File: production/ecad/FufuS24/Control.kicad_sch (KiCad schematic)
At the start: 28 parts, among them IC1 NLVPCA9535EDTR2G, J2 Conn_01x02, U1 RP2040, U2 W25Q128JVS

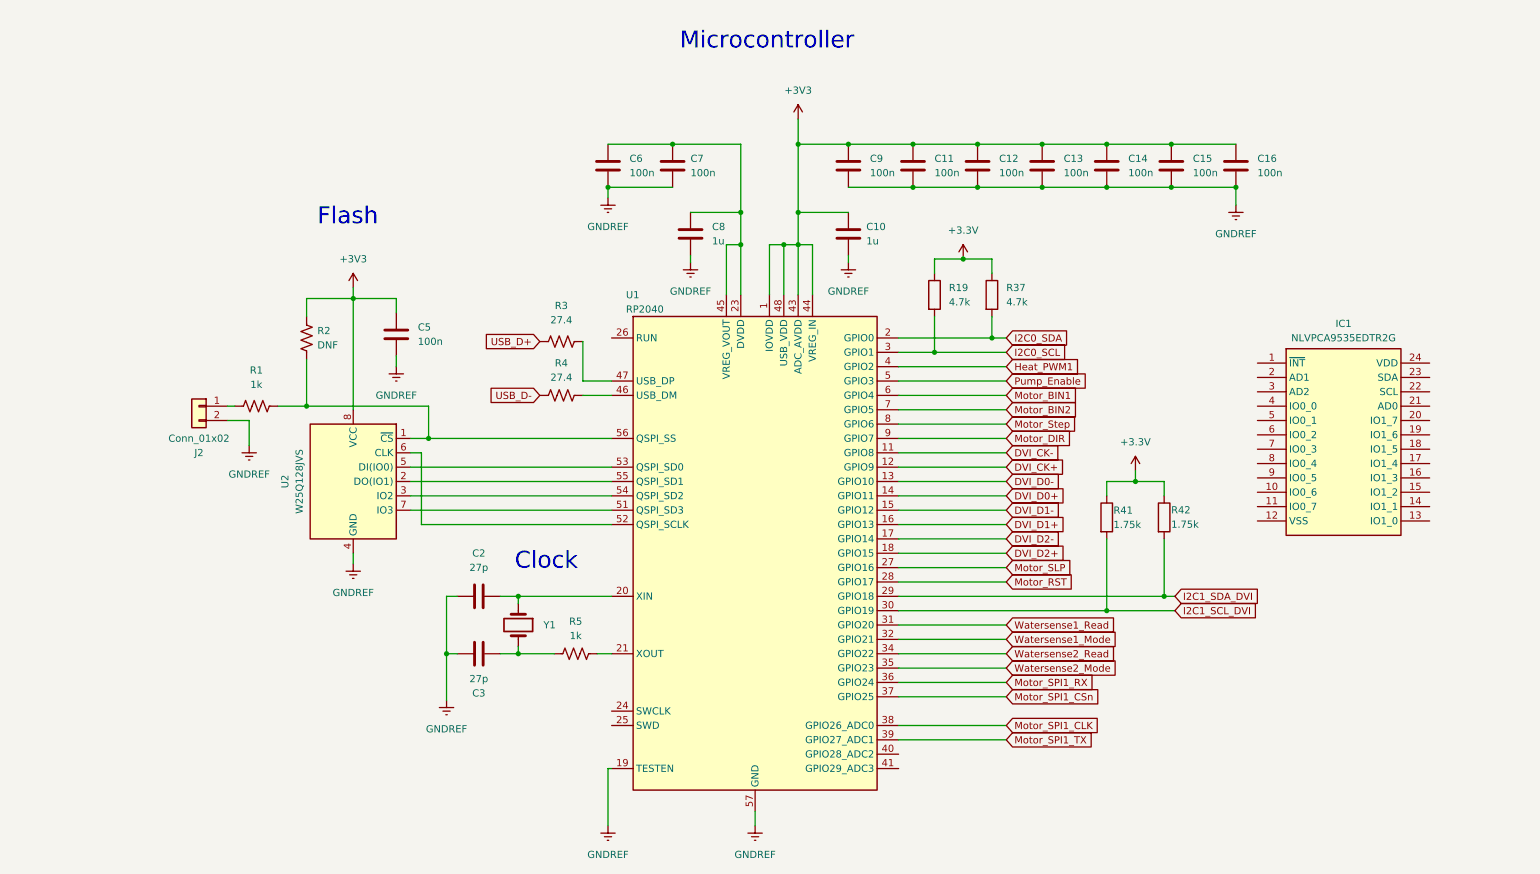
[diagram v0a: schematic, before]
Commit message: efan 2
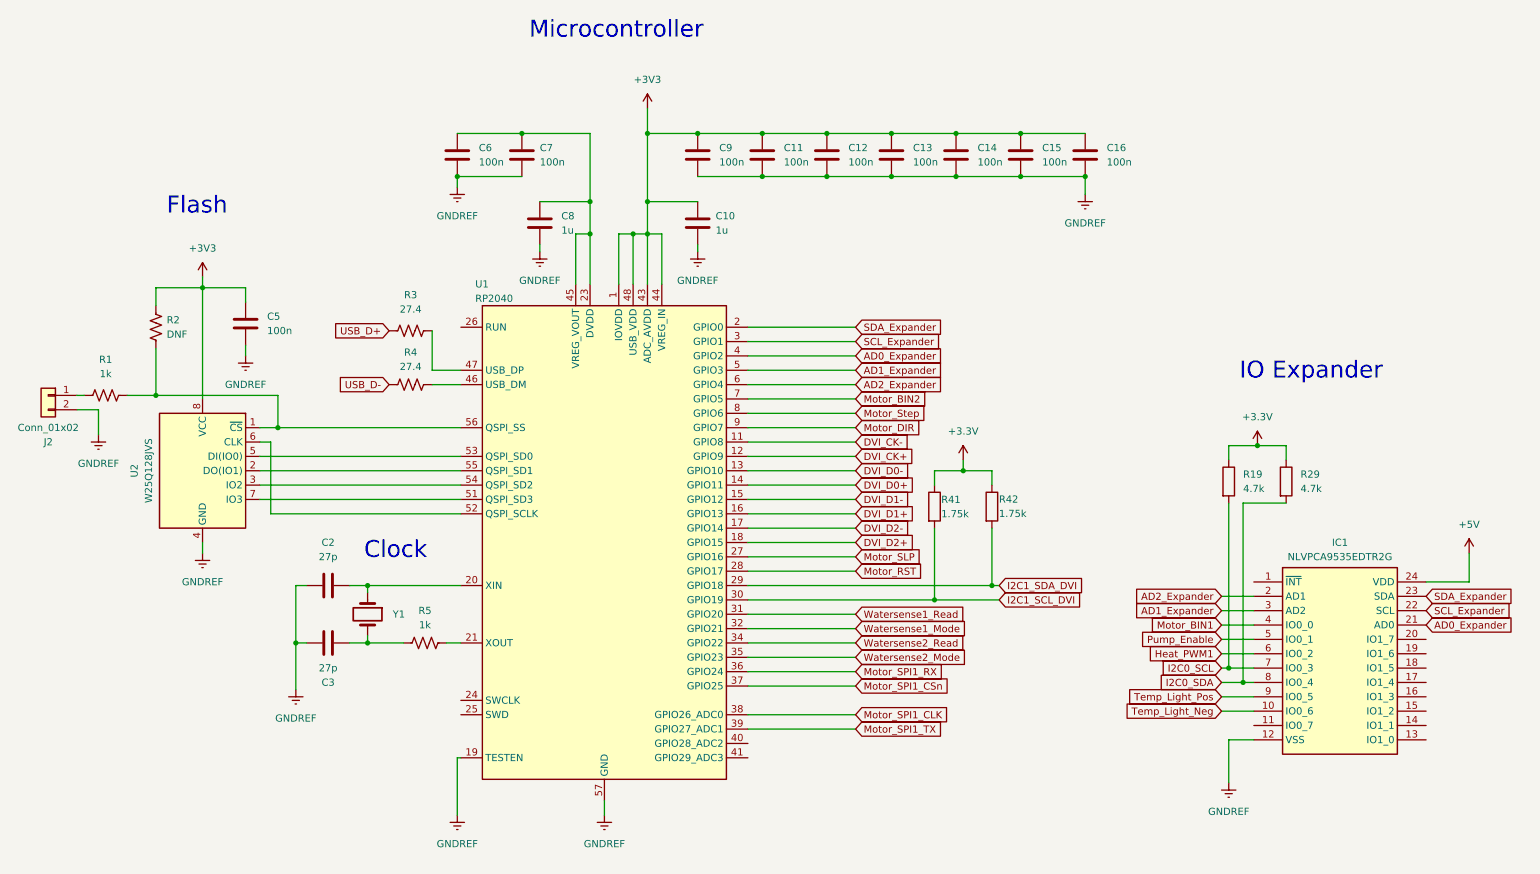
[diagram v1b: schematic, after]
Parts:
- removed R37: 4.7k, symbol Device:R
- added R29: 4.7k, symbol Device:R
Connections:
- net +3.3V: now also R29.1
- net GNDREF: now also IC1.12 (VSS)
- net Heat_PWM1: now also IC1.6 (IO0_2); no longer U1.4 (GPIO2)
- net I2C0_SCL: now also IC1.7 (IO0_3); no longer U1.3 (GPIO1)
- net I2C0_SDA: now also IC1.8 (IO0_4), R29.2; no longer U1.2 (GPIO0)
- net Motor_BIN1: now also IC1.4 (IO0_0); no longer U1.6 (GPIO4)
- net Pump_Enable: now also IC1.5 (IO0_1); no longer U1.5 (GPIO3)
- net Temp_Light_Neg: now reaches IC1.10 (IO0_6)
- net AD2_Expander: now reaches IC1.2 (AD1)
- net AD2_Expander: now also U1.6 (GPIO4)
- net AD0_Expander: now reaches IC1.21 (AD0)
- net AD0_Expander: now also U1.4 (GPIO2)
- net SCL_Expander: now reaches IC1.22 (SCL)
- net SCL_Expander: now also U1.3 (GPIO1)
- net SDA_Expander: now reaches IC1.23 (SDA)
- net SDA_Expander: now also U1.2 (GPIO0)
- net +5V: now reaches IC1.24 (VDD)
- net AD1_Expander: now reaches IC1.3 (AD2)
- net AD1_Expander: now also U1.5 (GPIO3)
- net Temp_Light_Pos: now reaches IC1.9 (IO0_5)
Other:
- note added: "IO Expander"
- moved on the sheet: C10, C11, C12, C13, C14, C15, C16, C2, C3, C5, C6, C7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

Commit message: efan 3
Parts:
- C10, C11, C12, C13, C14, C15, C16, C2, C3, C5, C6, C7, C8, C9: footprint (none) -> footprints:CAPC2012X94N
- IC1: footprint SOP65P640X120-24N -> footprints:SOP65P640X120-24N
- R1, R19, R2, R29, R3, R4, R41, R42, R5: footprint (none) -> footprints:RESC2012X60N
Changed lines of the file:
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@@
       (effects (font (size 1.27 1.27)))
     )
-    (property "Footprint" "SOP65P640X120-24N" (at 260.985 213.03 0)
+    (property "Footprint" "footprints:SOP65P640X120-24N" (at 260.985 213.03 0)
       (effects (font (size 1.27 1.27)) (justify left top) hide)
     )
@@
       (effects (font (size 1.27 1.27)) (justify left))
     )
-    (property "Footprint" "" (at 176.022 104.775 90)
+    (property "Footprint" "footprints:RESC2012X60N" (at 176.022 104.775 90)
       (effects (font (size 1.27 1.27)) hide)
     )
@@
       (effects (font (size 1.27 1.27)))
     )
-    (property "Footprint" "" (at 31.369 84.074 90)
+    (property "Footprint" "footprints:RESC2012X60N" (at 31.369 84.074 90)
       (effects (font (size 1.27 1.27)) hide)
     )
@@
       (effects (font (size 1.27 1.27)) (justify left))
     )
-    (property "Footprint" "" (at 159.7152 46.355 0)
+    (property "Footprint" "footprints:CAPC2012X94N" (at 159.7152 46.355 0)
       (effects (font (size 1.27 1.27)) hide)
     )
@@
       (effects (font (size 1.27 1.27)) (justify left))
     )
-    (property "Footprint" "" (at 105.7402 46.355 0)
+    (property "Footprint" "footprints:CAPC2012X94N" (at 105.7402 46.355 0)
       (effects (font (size 1.27 1.27)) hide)
     )
@@
       (effects (font (size 1.27 1.27)) (justify left))
     )
-    (property "Footprint" "" (at 186.182 104.775 90)
+    (property "Footprint" "footprints:RESC2012X60N" (at 186.182 104.775 90)
       (effects (font (size 1.27 1.27)) hide)
     )
@@
       (effects (font (size 1.27 1.27)) (justify left))
     )
-    (property "Footprint" "" (at 205.4352 46.355 0)
+    (property "Footprint" "footprints:CAPC2012X94N" (at 205.4352 46.355 0)
       (effects (font (size 1.27 1.27)) hide)
     )
@@
       (effects (font (size 1.27 1.27)) (justify left))
     )
-    (property "Footprint" "" (at 171.1452 46.355 0)
+    (property "Footprint" "footprints:CAPC2012X94N" (at 171.1452 46.355 0)
       (effects (font (size 1.27 1.27)) hide)
     )
@@
       (effects (font (size 1.27 1.27)))
     )
-    (property "Footprint" "" (at 87.884 127.889 90)
+    (property "Footprint" "footprints:RESC2012X60N" (at 87.884 127.889 90)
       (effects (font (size 1.27 1.27)) hide)
     )
@@
       (effects (font (size 1.27 1.27)) (justify left))
     )
-    (property "Footprint" "" (at 56.8452 76.2 0)
+    (property "Footprint" "footprints:CAPC2012X94N" (at 56.8452 76.2 0)
       (effects (font (size 1.27 1.27)) hide)
     )
@@
       (effects (font (size 1.27 1.27)))
     )
-    (property "Footprint" "" (at 85.344 72.644 90)
+    (property "Footprint" "footprints:RESC2012X60N" (at 85.344 72.644 90)
       (effects (font (size 1.27 1.27)) hide)
     )
@@
       (effects (font (size 1.27 1.27)) (justify left))
     )
-    (property "Footprint" "" (at 182.5752 46.355 0)
+    (property "Footprint" "footprints:CAPC2012X94N" (at 182.5752 46.355 0)
       (effects (font (size 1.27 1.27)) hide)
     )
@@
       (effects (font (size 1.27 1.27)))
     )
-    (property "Footprint" "" (at 85.344 82.169 90)
+    (property "Footprint" "footprints:RESC2012X60N" (at 85.344 82.169 90)
       (effects (font (size 1.27 1.27)) hide)
     )
@@
       (effects (font (size 1.27 1.27)) (justify left))
     )
-    (property "Footprint" "" (at 136.8552 58.42 0)
+    (property "Footprint" "footprints:CAPC2012X94N" (at 136.8552 58.42 0)
       (effects (font (size 1.27 1.27)) hide)
     )
@@
       (effects (font (size 1.27 1.27)) (justify right))
     )
-    (property "Footprint" "" (at 38.989 72.771 90)
+    (property "Footprint" "footprints:RESC2012X60N" (at 38.989 72.771 90)
       (effects (font (size 1.27 1.27)) hide)
     )
@@
       (effects (font (size 1.27 1.27)))
     )
-    (property "Footprint" "" (at 74.295 117.7798 0)
+    (property "Footprint" "footprints:CAPC2012X94N" (at 74.295 117.7798 0)
       (effects (font (size 1.27 1.27)) hide)
     )
@@
       (effects (font (size 1.27 1.27)) (justify left))
     )
-    (property "Footprint" "" (at 238.252 100.33 90)
+    (property "Footprint" "footprints:RESC2012X60N" (at 238.252 100.33 90)
       (effects (font (size 1.27 1.27)) hide)
     )
@@
       (effects (font (size 1.27 1.27)) (justify left))
     )
-    (property "Footprint" "" (at 108.9152 58.42 0)
+    (property "Footprint" "footprints:CAPC2012X94N" (at 108.9152 58.42 0)
       (effects (font (size 1.27 1.27)) hide)
     )
@@
       (effects (font (size 1.27 1.27)) (justify left))
     )
-    (property "Footprint" "" (at 94.3102 46.355 0)
+    (property "Footprint" "footprints:CAPC2012X94N" (at 94.3102 46.355 0)
       (effects (font (size 1.27 1.27)) hide)
     )
@@
       (effects (font (size 1.27 1.27)) (justify left))
     )
-    (property "Footprint" "" (at 194.0052 46.355 0)
+    (property "Footprint" "footprints:CAPC2012X94N" (at 194.0052 46.355 0)
       (effects (font (size 1.27 1.27)) hide)
     )
@@
       (effects (font (size 1.27 1.27)) (justify left))
     )
-    (property "Footprint" "" (at 136.8552 46.355 0)
+    (property "Footprint" "footprints:CAPC2012X94N" (at 136.8552 46.355 0)
       (effects (font (size 1.27 1.27)) hide)
     )
@@
       (effects (font (size 1.27 1.27)) (justify left))
     )
-    (property "Footprint" "" (at 228.092 100.33 90)
+    (property "Footprint" "footprints:RESC2012X60N" (at 228.092 100.33 90)
       (effects (font (size 1.27 1.27)) hide)
     )
@@
       (effects (font (size 1.27 1.27)) (justify left))
     )
-    (property "Footprint" "" (at 148.2852 46.355 0)
+    (property "Footprint" "footprints:CAPC2012X94N" (at 148.2852 46.355 0)
       (effects (font (size 1.27 1.27)) hide)
     )
@@
       (effects (font (size 1.27 1.27)))
     )
-    (property "Footprint" "" (at 74.295 129.8702 0)
-      (effects (font (size 1.27 1.27)) hide)
-    )
+    (property "Footprint" "footprints:CAPC2012X94N" (at 74.295 129.8702 0)
+      (effects (font (size 1.27 1.27)) hide)
+    )
